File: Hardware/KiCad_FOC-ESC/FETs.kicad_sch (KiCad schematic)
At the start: 6 parts, among them Q1 NTTFS5D6N08XLTAG, Q2 NTTFS5D6N08XLTAG, Q3 NTTFS5D6N08XLTAG, Q4 NTTFS5D6N08XLTAG, Q5 NTTFS5D6N08XLTAG, Q6 NTTFS5D6N08XLTAG

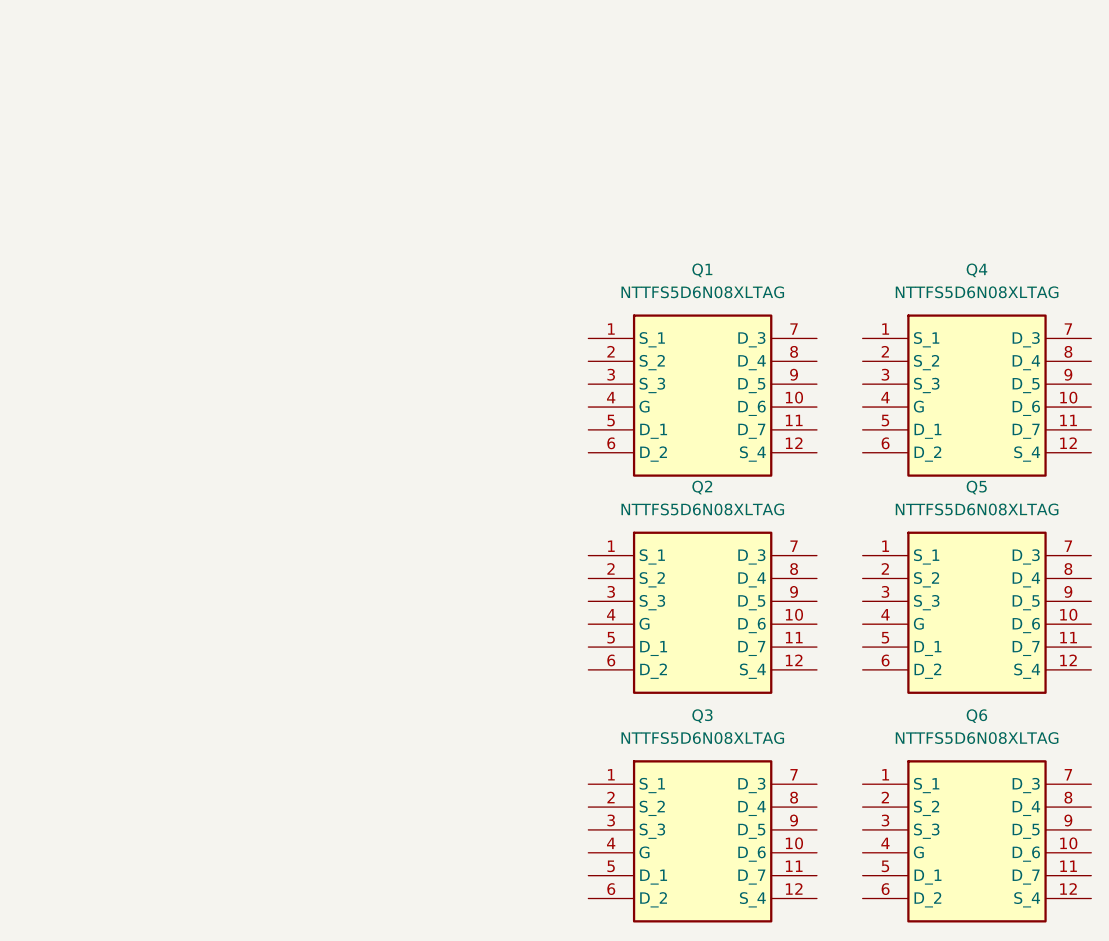
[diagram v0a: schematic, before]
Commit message: updated:schematics (#9)
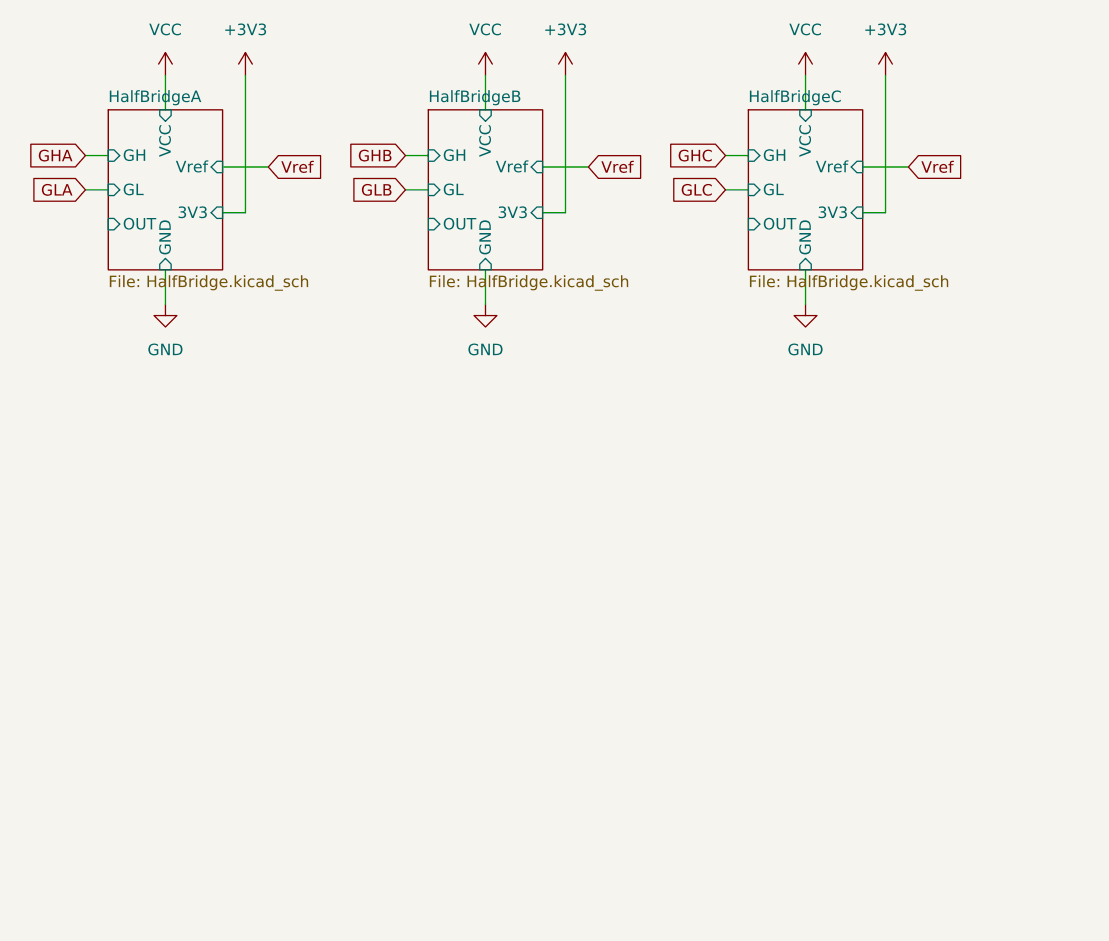
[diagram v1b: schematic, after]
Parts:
- removed Q1, Q2, Q3, Q4, Q5, Q6: NTTFS5D6N08XLTAG, SamacSys_Parts:NVTFS007N08HLTAG, symbol SamacSys_Parts:NTTFS5D6N08XLTAG
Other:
- added sheet HalfBridgeA (HalfBridge.kicad_sch)
- added sheet HalfBridgeB (HalfBridge.kicad_sch)
- added sheet HalfBridgeC (HalfBridge.kicad_sch)
